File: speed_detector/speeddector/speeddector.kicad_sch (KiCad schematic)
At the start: 5 parts

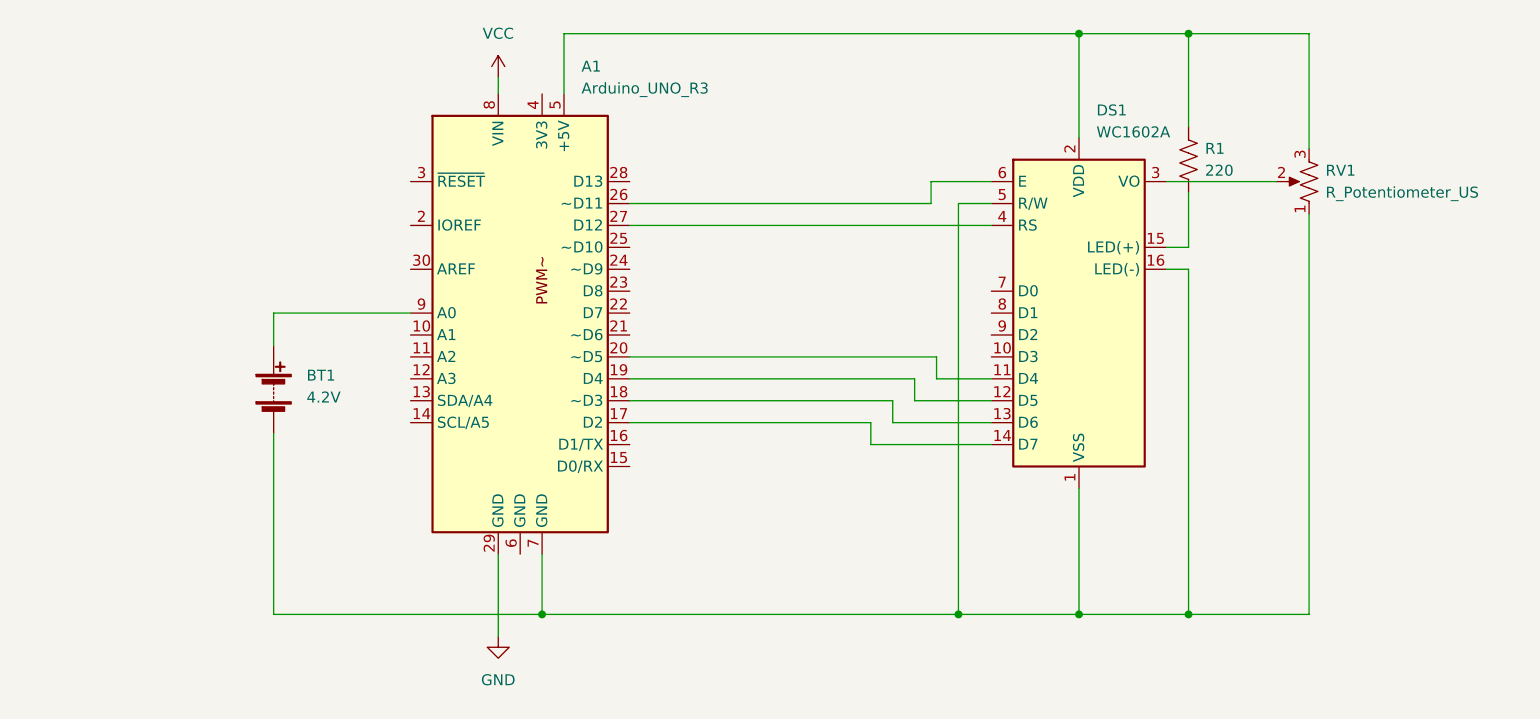
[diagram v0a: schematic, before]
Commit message: project with ir sensor
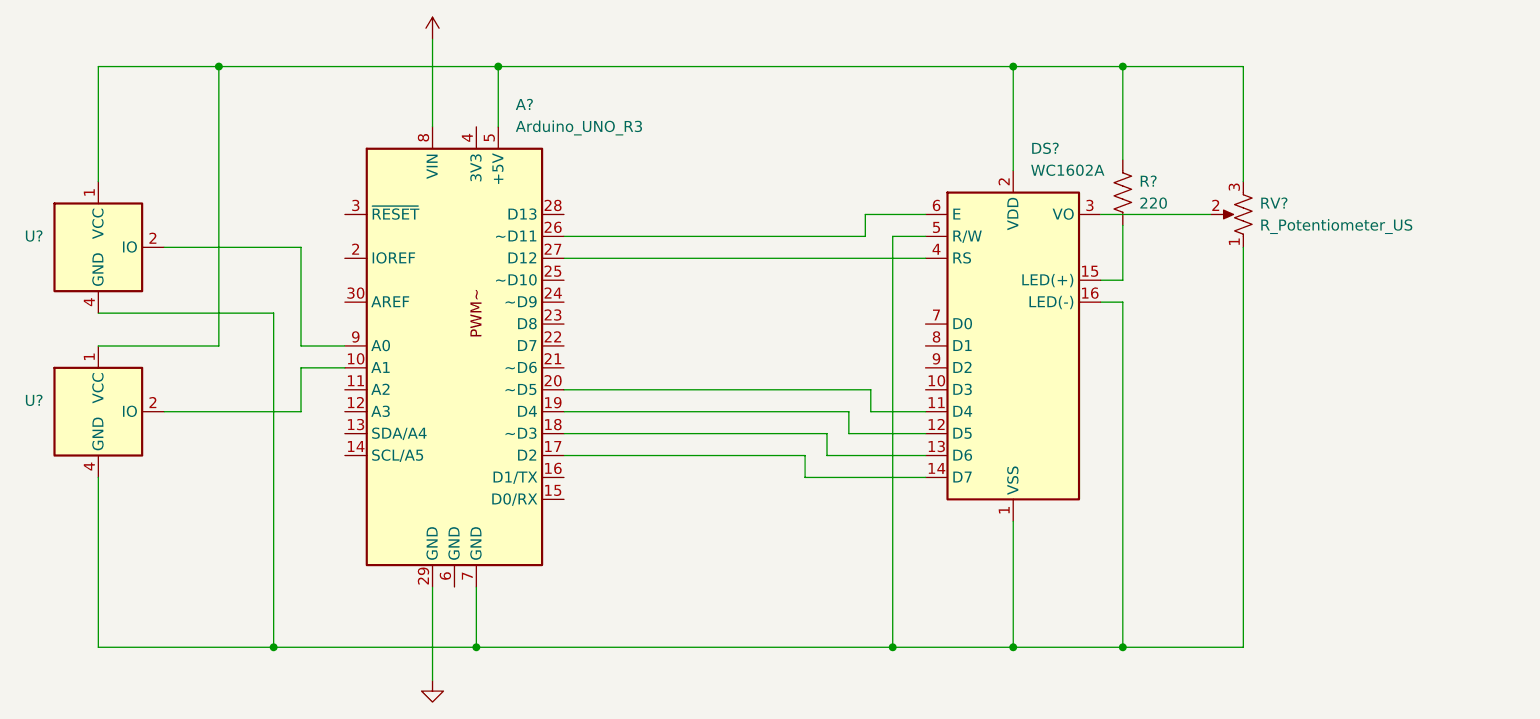
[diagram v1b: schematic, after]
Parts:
- removed A1: Arduino_UNO_R3, Module:Arduino_UNO_R3, symbol Arduino:Arduino_UNO_R3
- removed BT1: 4.2V, symbol Device:Battery
- removed DS1: WC1602A, Display:WC1602A, symbol Display_Character:WC1602A
- removed R1: 220, symbol Device:R_US
- removed RV1: R_Potentiometer_US, symbol Device:R_Potentiometer_US
- added A?: Arduino_UNO_R3, Module:Arduino_UNO_R3, symbol Arduino:Arduino_UNO_R3
- added DS?: WC1602A, Display:WC1602A, symbol Display_Character:WC1602A
- added R?: 220, symbol Device:R_US
- added RV?: R_Potentiometer_US, symbol Device:R_Potentiometer_US
- added U? (x2): (no value), symbol Sensor:DHT11
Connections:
- net GND: now also A?.29 (GND)
- net VCC: now also A?.8 (VIN)
- new net: A?.7 (GND), DS?.1 (VSS), DS?.16 (LED(-)), DS?.5 (R/W), RV?.1, U?.4 (GND), U?.4 (GND)
- new net: DS?.3 (VO), RV?.2
- new net: A?.5 (+5V), DS?.2 (VDD), R?.1, RV?.3, U?.1 (VCC), U?.1 (VCC)
- new net: A?.10 (A1), U?.2 (IO)
- new net: A?.17 (D2), DS?.14 (D7)
- new net: A?.18 (~D3), DS?.13 (D6)
- new net: A?.19 (D4), DS?.12 (D5)
- new net: A?.20 (~D5), DS?.11 (D4)
- new net: A?.26 (~D11), DS?.6 (E)
- new net: A?.27 (D12), DS?.4 (RS)
- new net: A?.9 (A0), U?.2 (IO)
- new net: DS?.15 (LED(+)), R?.2
